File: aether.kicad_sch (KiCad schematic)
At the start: 41 parts, among them Q1 NPN, Q2 CSD17575Q3, Q3 CSD17575Q3, Q4 CSD17575Q3, Q5 CSD17575Q3, SW1 TDD01H0SB1R, U1 USBLC6-2SC6

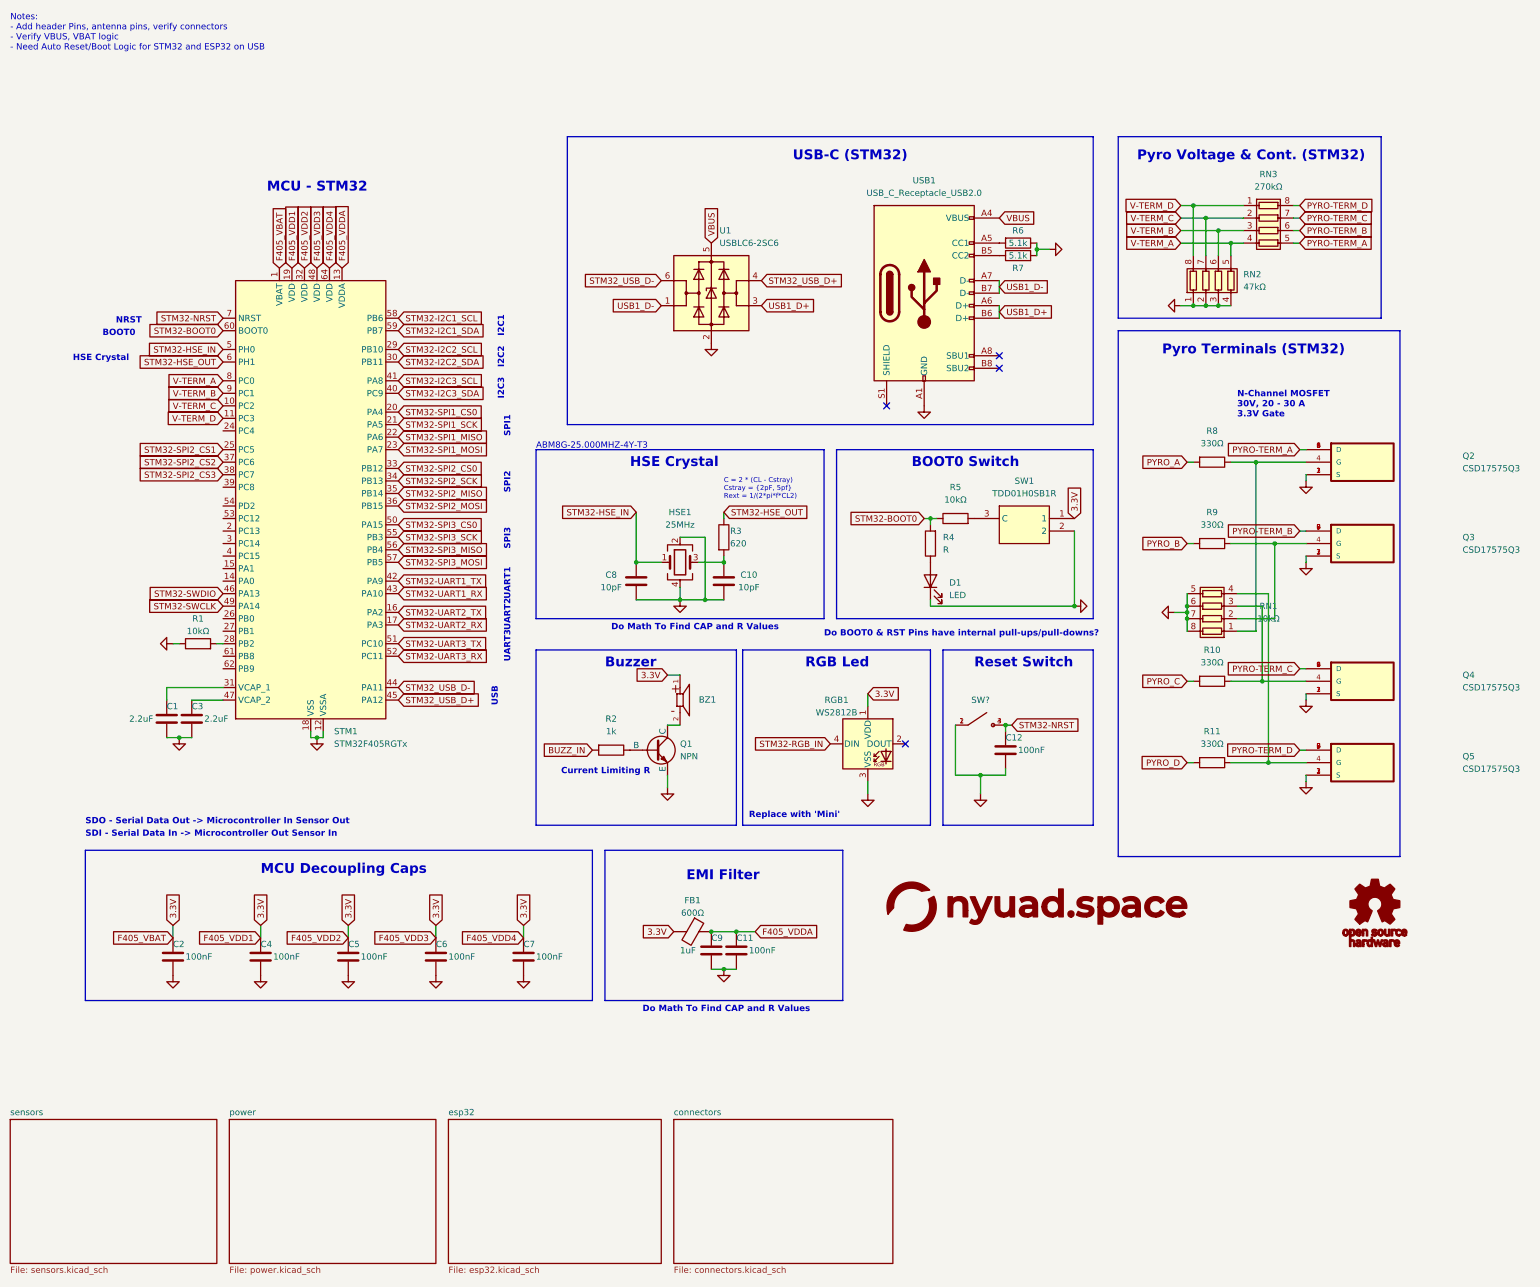
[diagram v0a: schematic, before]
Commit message: significant amount of routing done
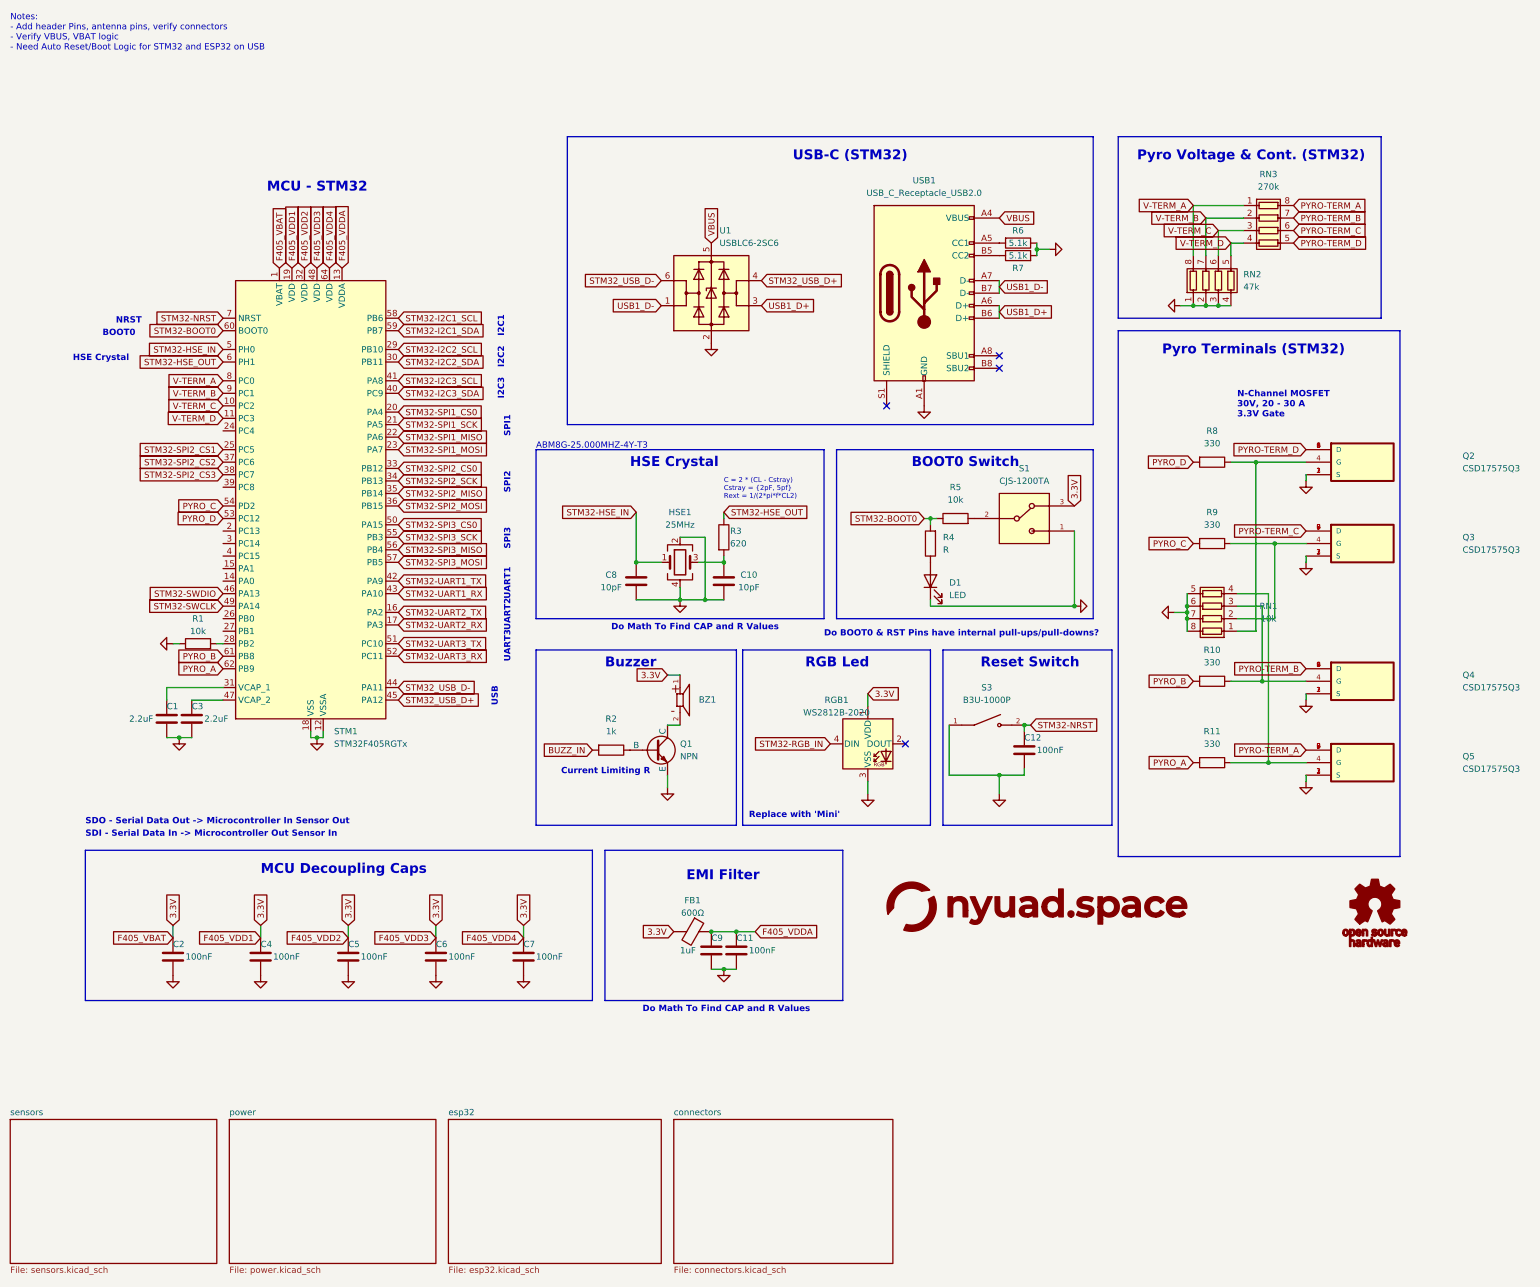
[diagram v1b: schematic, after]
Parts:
- removed SW1: TDD01H0SB1R, TDD01H0SB1R:SOT175P420X230-3N, symbol TDD01H0SB1R:TDD01H0SB1R
- removed SW?: PTS526_SM08_SMTR2_LFS, PTS526_SM08_SMTR2_LFS:SW_PTS526_SM08_SMTR2_LFS, symbol PTS526_SM08_SMTR2_LFS:PTS526_SM08_SMTR2_LFS
- added S1: CJS-1200TA, CJS-1200TA:SW_CJS-1200TA, symbol CJS-1200TA:CJS-1200TA
- added S3: B3U-1000P, B3U-1000P:SW_B3U-1000P, symbol B3U-1000P:B3U-1000P
- D1: footprint LED_SMD:LED_0603_1608Metric -> LED_SMD:LED_0402_1005Metric
- R1, R5: value 10kΩ -> 10k; footprint Resistor_SMD:R_0603_1608Metric -> Resistor_SMD:R_0402_1005Metric
- R10, R11, R8, R9: value 330Ω -> 330
- R2, R3, R4, R6, R7: footprint Resistor_SMD:R_0603_1608Metric -> Resistor_SMD:R_0402_1005Metric
- RGB1: value WS2812B -> WS2812B-2020; footprint LED_SMD:LED_WS2812B_PLCC4_5.0x5.0mm_P3.2mm -> LED_SMD:LED_WS2812B-2020_PLCC4_2.0x2.0mm
- RN1: value 10kΩ -> 10k
- RN2: value 47kΩ -> 47k
- RN3: value 270kΩ -> 270k
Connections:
- net 3.3V: now also S1.3
- net GND: now also S1.1, S3.1
- net PYRO-TERM_A: now also Q5.5 (D), Q5.6 (D), Q5.7 (D), Q5.8 (D), Q5.9 (D), RN3.8 (R1.2); no longer Q2.5 (D), Q2.6 (D), Q2.7 (D), Q2.8 (D), Q2.9 (D), RN3.5 (R4.2)
- net PYRO-TERM_B: now also Q4.5 (D), Q4.6 (D), Q4.7 (D), Q4.8 (D), Q4.9 (D), RN3.7 (R2.2); no longer Q3.5 (D), Q3.6 (D), Q3.7 (D), Q3.8 (D), Q3.9 (D), RN3.6 (R3.2)
- net PYRO-TERM_C: now also Q3.5 (D), Q3.6 (D), Q3.7 (D), Q3.8 (D), Q3.9 (D), RN3.6 (R3.2); no longer Q4.5 (D), Q4.6 (D), Q4.7 (D), Q4.8 (D), Q4.9 (D), RN3.7 (R2.2)
- net PYRO-TERM_D: now also Q2.5 (D), Q2.6 (D), Q2.7 (D), Q2.8 (D), Q2.9 (D), RN3.5 (R4.2); no longer Q5.5 (D), Q5.6 (D), Q5.7 (D), Q5.8 (D), Q5.9 (D), RN3.8 (R1.2)
- net PYRO_A: now also R11.2, STM1.62 (PB9); no longer R8.2
- net PYRO_B: now also R10.2, STM1.61 (PB8); no longer R9.2
- net PYRO_C: now also R9.2, STM1.54 (PD2); no longer R10.2
- net PYRO_D: now also R8.2, STM1.53 (PC12); no longer R11.2
- net STM32-NRST: now also S3.2
- net V-TERM_A: now also RN2.8 (R1.2), RN3.1 (R1.1); no longer RN2.5 (R4.2), RN3.4 (R4.1)
- net V-TERM_B: now also RN2.7 (R2.2), RN3.2 (R2.1); no longer RN2.6 (R3.2), RN3.3 (R3.1)
- net V-TERM_C: now also RN2.6 (R3.2), RN3.3 (R3.1); no longer RN2.7 (R2.2), RN3.2 (R2.1)
- net V-TERM_D: now also RN2.5 (R4.2), RN3.4 (R4.1); no longer RN2.8 (R1.2), RN3.1 (R1.1)
- net at R5.2: now also S1.2
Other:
- moved on the sheet: C12
